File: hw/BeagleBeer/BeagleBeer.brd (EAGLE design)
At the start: 130.8 x 118.7 mm, 104 parts, among them Q10 BSS138, Q9 BSS138, U1 TEMPERATURE-SENSORUMAX8, U4 CAT24C256WI-GT3, U5 BEAGLEBONE_OUTLINEBEAGLEBEER

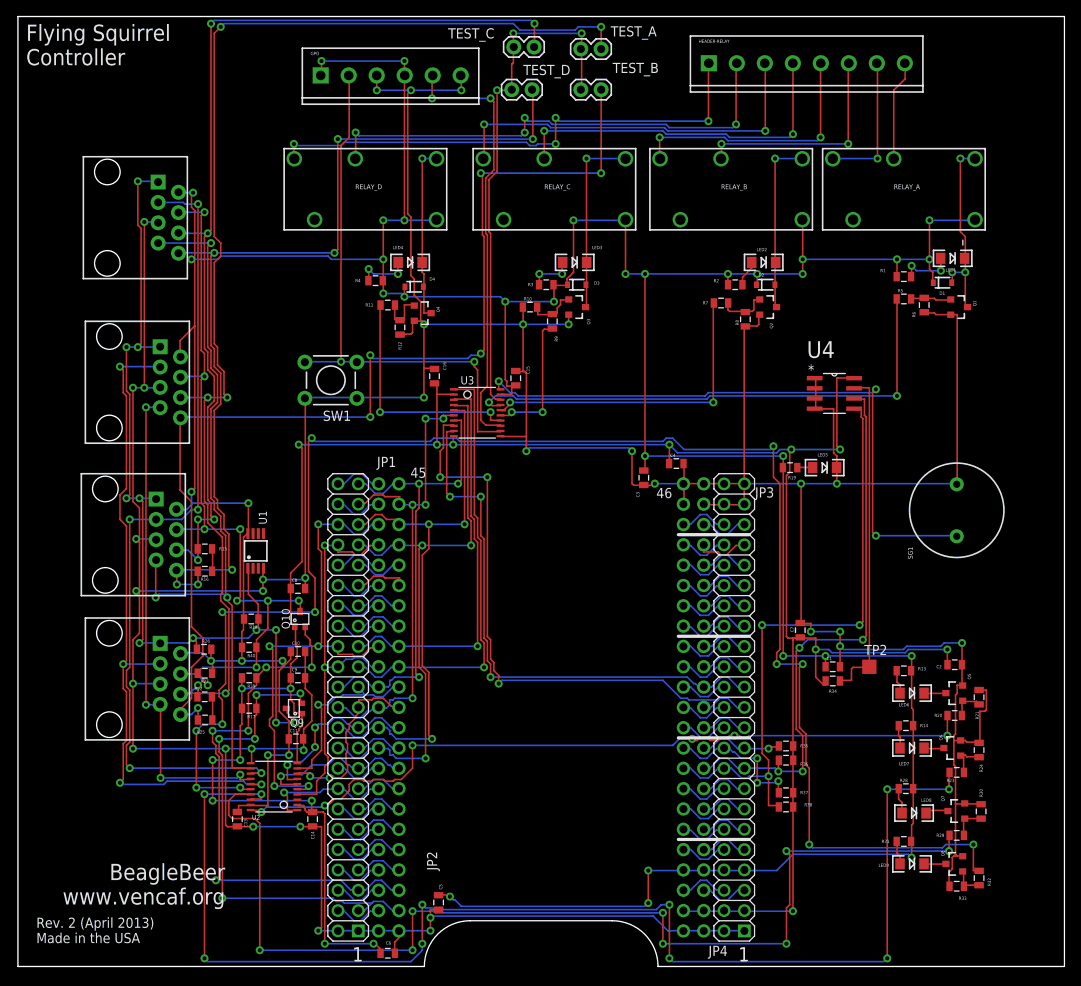
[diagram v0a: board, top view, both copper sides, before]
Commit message: BeagleBeer v2 Run ERCs and DRCs
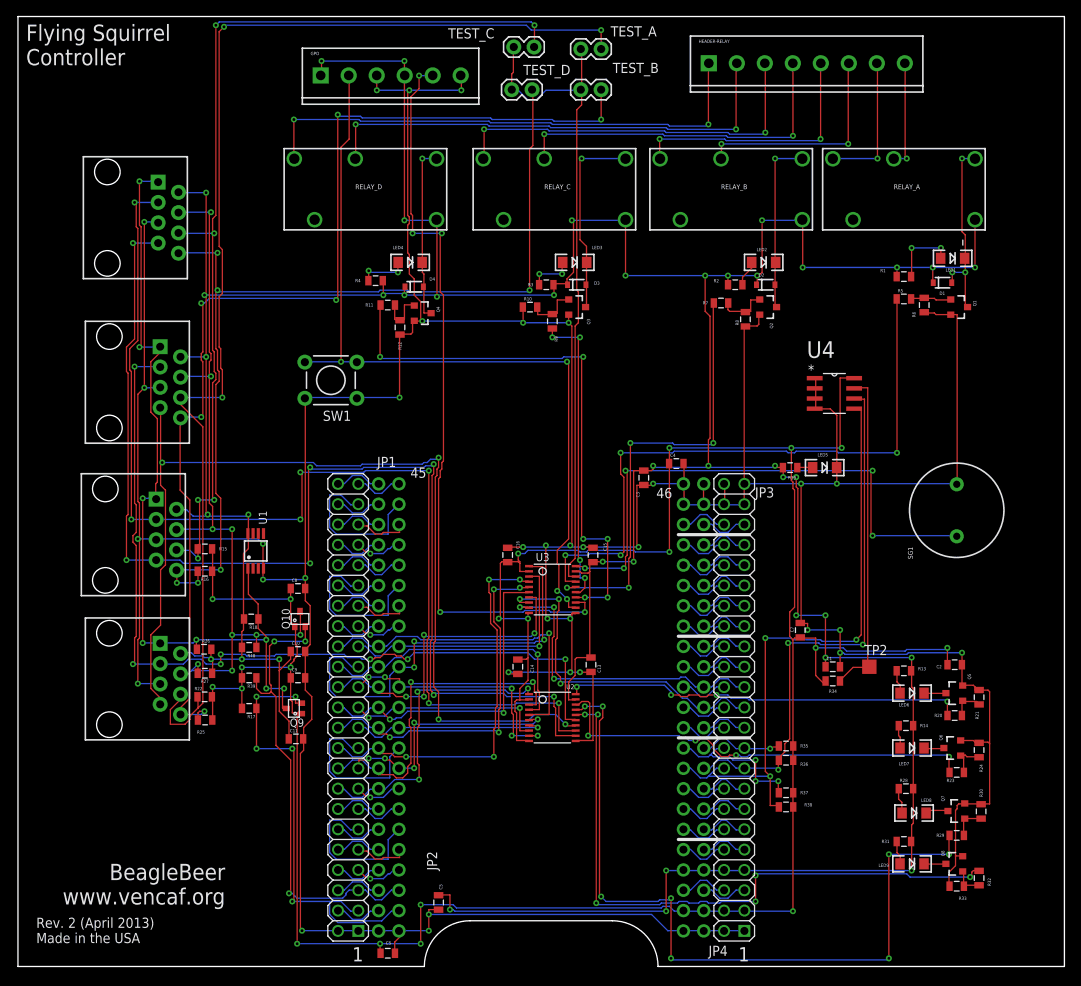
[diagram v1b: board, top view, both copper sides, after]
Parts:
- moved C13 48.2 mm to (71.7, 37.7)
- moved U2 35.9 mm to (66.9, 31.1), turned to 270 degrees
- moved C14 32.0 mm to (62.5, 37.5)
- moved C16 24.2 mm to (61.3, 51.4)
- moved C15 24.1 mm to (71.9, 51.4)
- moved U3 24.0 mm to (66.9, 47.1)
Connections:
- new net N$12: JP2.20, U5.40
- new net N$13: JP2.21, U5.42
- new net N$20: JP1.4, U5.39
- new net N$21: JP1.3, U5.41
- net 3.3V: now also R15.2, R16.2, R22.2, R25.2
- net LED_FLOW_B_3P3: now also U2.3
- net LED_FLOW_C_3P3: no longer JP2.20, U5.40
- net LED_FLOW_D_3P3: no longer JP2.21, U5.42
- net N$2: now also JP1.2, U5.43; no longer R22.2, R25.2
- net N$3: now also JP1.1, U5.45; no longer R15.2, R16.2
- net RELAY_A_3P3: no longer JP1.4, U5.39
- net RELAY_B_3P3: no longer JP1.3, U5.41
- net RELAY_C_3P3: no longer JP1.2, U5.43
- net RELAY_D_3P3: no longer JP1.1, U5.45
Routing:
- net LED_FLOW_D: track 204.4 -> 79.0 mm, vias 12 -> 6
- net LED_FLOW_B: track 159.9 -> 55.1 mm, vias 10 -> 4
- net GPIO_B: track 62.0 -> 125.5 mm
- net GPIO_D: track 90.7 -> 146.5 mm, vias 3 -> 7
- net LED_FLOW_A: track 96.8 -> 50.6 mm, vias 6 -> 4
- net ALARM: track 54.3 -> 94.1 mm, vias 2 -> 5
- net RELAY_D: track 29.5 -> 69.3 mm, vias 2 -> 6
- net LED_FLOW_C: track 133.9 -> 94.6 mm
- net 3.3V: track 304.1 -> 339.9 mm, vias 17 -> 20
- net LED_FLOW_B_3P3: track 6.10 -> 41.8 mm, vias 0 -> 2
- net GPIO_C: track 102.1 -> 137.8 mm, vias 5 -> 7
- net RESET: track 69.3 -> 102.2 mm, vias 2 -> 4
- net ALARM_3P3: track 75.1 -> 43.0 mm
- net RESET_3P3: track 69.4 -> 39.8 mm
- net RELAY_B_3P3: track 71.7 -> 45.2 mm, vias 3 -> 4
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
